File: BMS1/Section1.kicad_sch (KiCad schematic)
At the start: 68 parts

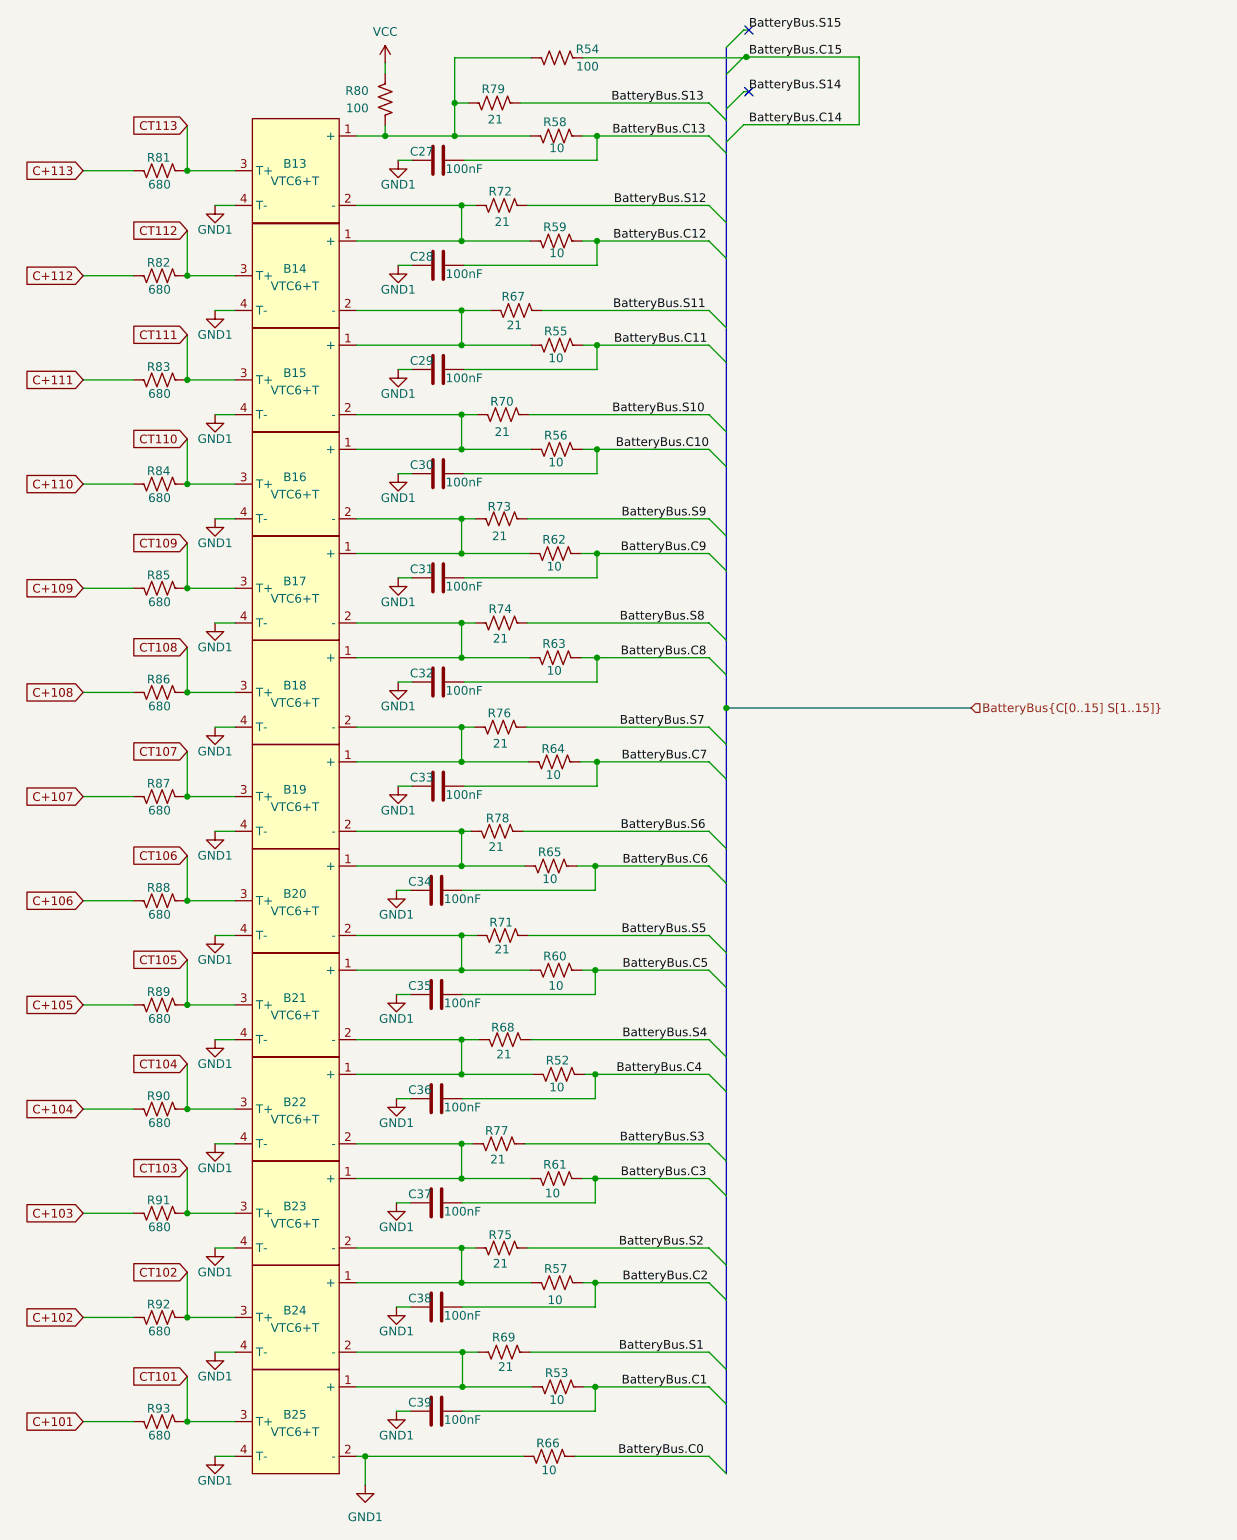
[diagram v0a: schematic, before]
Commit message: Cap Change
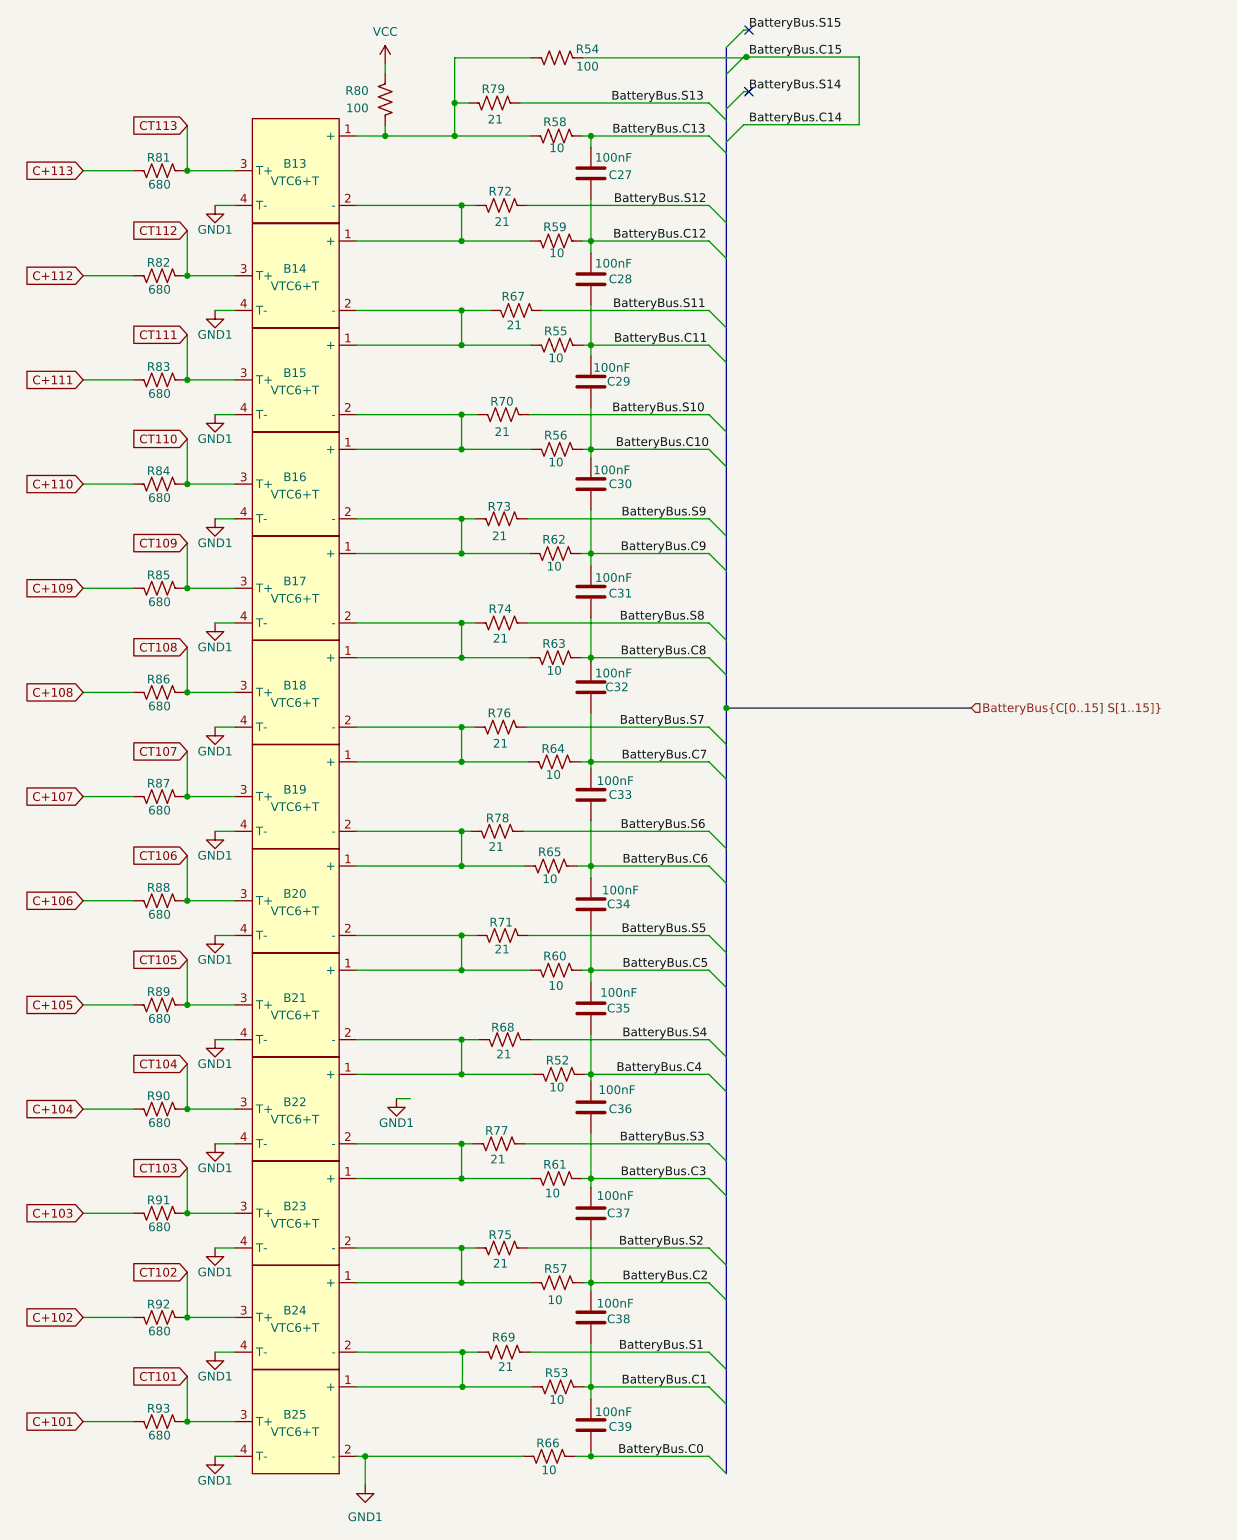
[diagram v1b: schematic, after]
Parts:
- R79: footprint Resistor_SMD:R_2512_6332Metric_Pad1.40x3.35mm_HandSolder -> Resistor_SMD:R_0603_1608Metric_Pad0.98x0.95mm_HandSolder
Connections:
- net BatteryBus.C0: now also C39.2
- net BatteryBus.C1: now also C38.2
- net BatteryBus.C10: now also C29.2
- net BatteryBus.C11: now also C28.2
- net BatteryBus.C12: now also C27.2
- net BatteryBus.C2: now also C37.2
- net BatteryBus.C3: now also C36.2
- net BatteryBus.C4: now also C35.2
- net BatteryBus.C5: now also C34.2
- net BatteryBus.C6: now also C33.2
- net BatteryBus.C7: now also C32.1
- net BatteryBus.C8: now also C31.2, C32.2; no longer C32.1
- net BatteryBus.C9: now also C30.2
- net GND1: no longer C27.2, C28.2, C29.2, C30.2, C31.2, C32.2, C33.2, C34.2, C35.2, C36.2, C37.2, C38.2, C39.2
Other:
- moved on the sheet: C27, C28, C29, C30, C31, C32, C33, C34, C35, C36, C37, C38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
